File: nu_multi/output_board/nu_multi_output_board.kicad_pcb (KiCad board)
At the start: 2 copper layers, 40 x 18 mm, 3 parts, among them J1 CONN_02X07, J2 CONN_02X05

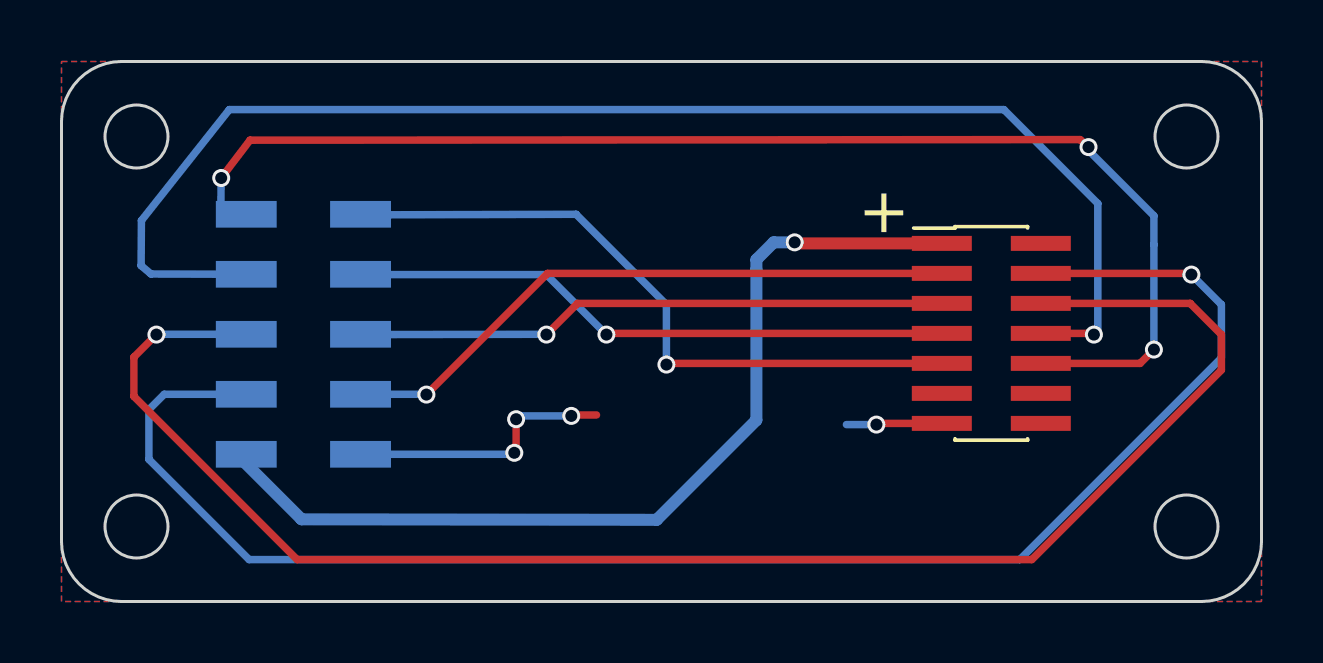
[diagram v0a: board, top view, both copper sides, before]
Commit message: Updated output board
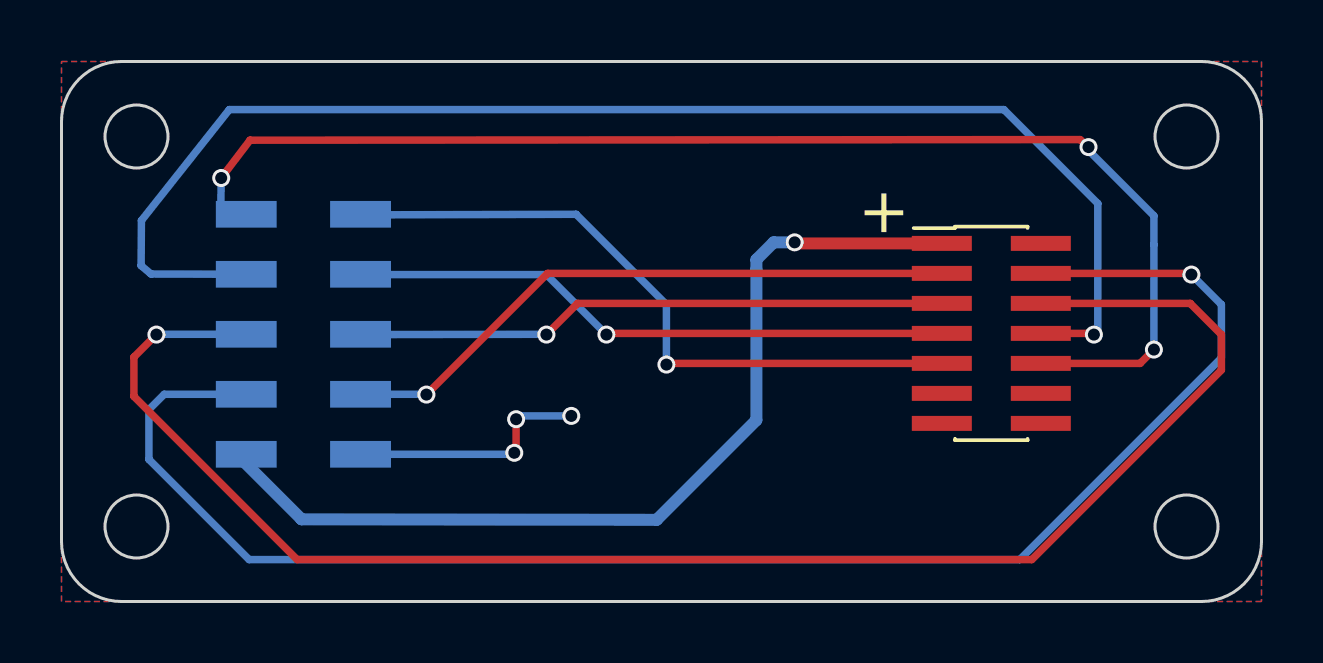
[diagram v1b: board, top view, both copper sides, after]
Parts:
- J1: value CONN_02X07 -> Conn_02x07_Odd_Even
- J2: value CONN_02X05 -> Conn_02x05_Odd_Even
- moved G*** 1.36 mm to (148.6, 65.1)
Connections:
- net Net-(J1-Pad1) renamed V+
- net Net-(J1-Pad10) renamed CH7
- net Net-(J1-Pad3) renamed CH2
- net Net-(J1-Pad4) renamed CH1
- net Net-(J1-Pad5) renamed CH4
- net Net-(J1-Pad6) renamed CH3
- net Net-(J1-Pad7) renamed CH6
- net Net-(J1-Pad8) renamed CH5
- net Net-(J1-Pad9) renamed CH8
- J1 pad 11: GND -> CH10
- J1 pad 12: GND -> CH9
- J1 pad 13: GND -> CH12
- J1 pad 14: GND -> CH11
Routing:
- net GND: track 12.2 -> 8.22 mm, vias 4 -> 3
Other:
- net class Default removed
- board text added: "Output Board 2.5.1"
